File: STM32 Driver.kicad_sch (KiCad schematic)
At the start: 16 parts, among them J4 USB_C_Receptacle_USB2.0_14P, U1 MCP1700x-330xxMB, U2 STM32F072C8Tx

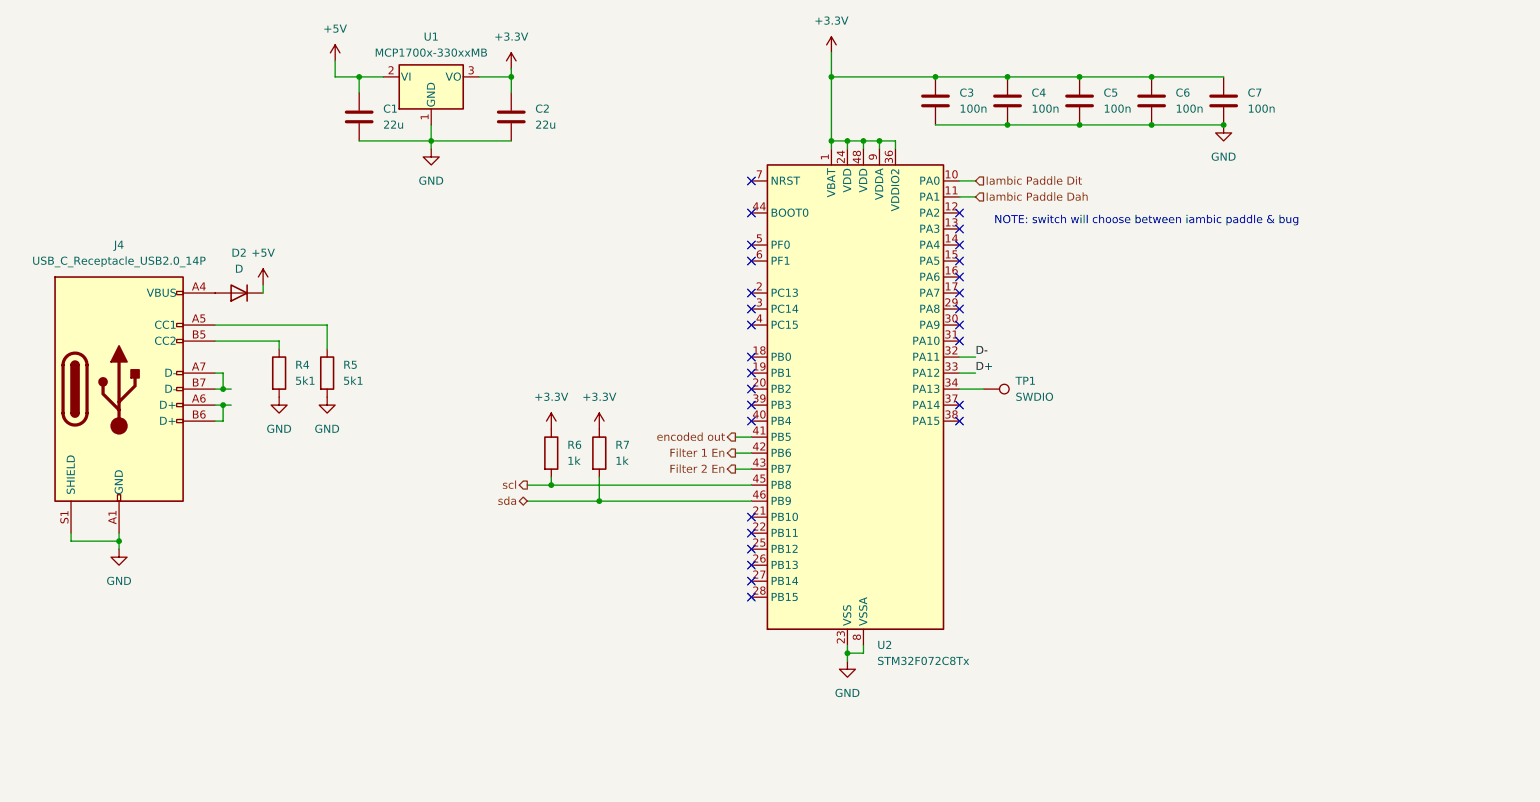
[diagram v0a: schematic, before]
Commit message: update
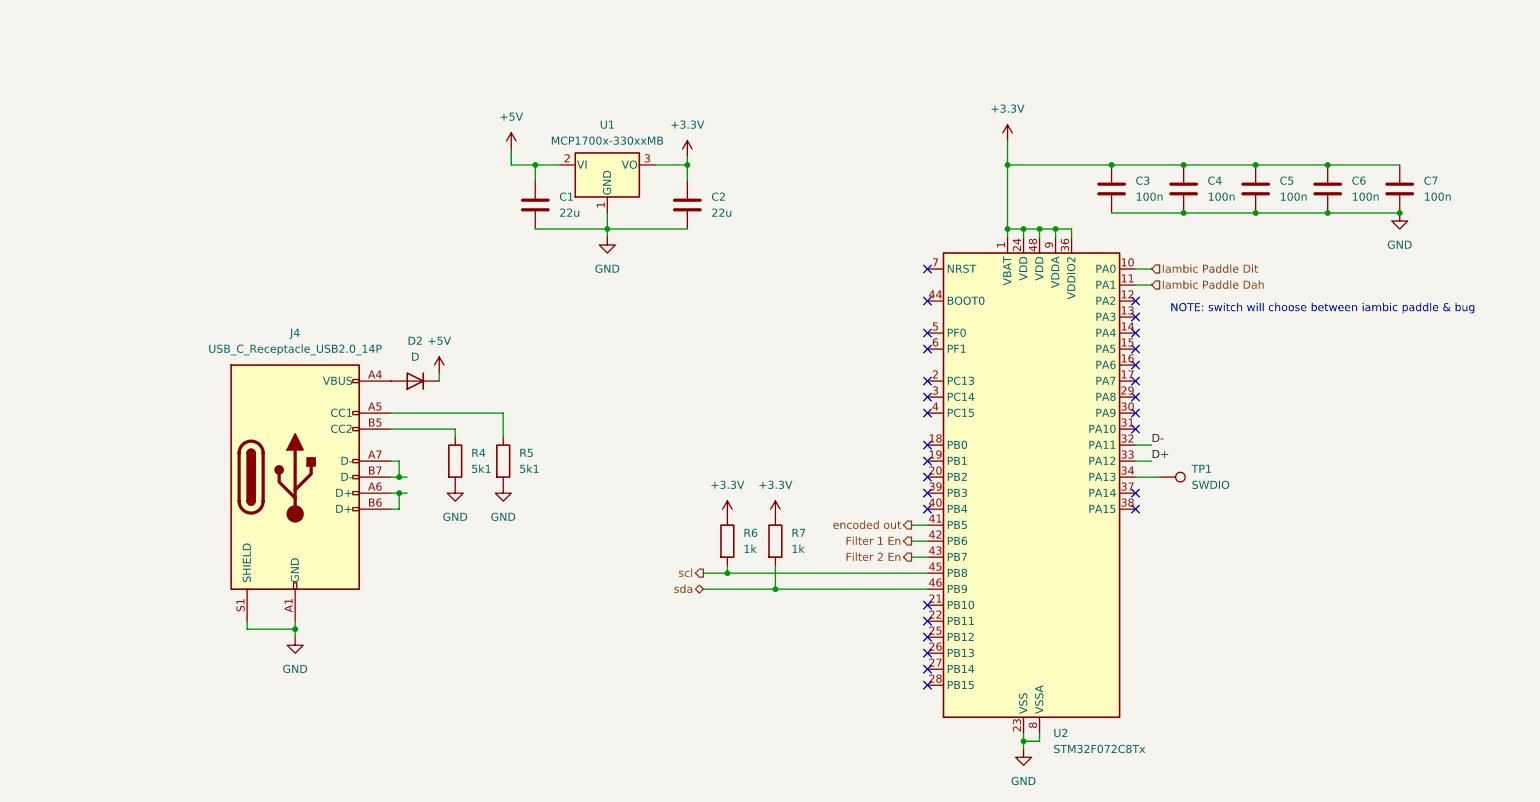
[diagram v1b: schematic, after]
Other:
- title: STM32 Driver -> (none)
